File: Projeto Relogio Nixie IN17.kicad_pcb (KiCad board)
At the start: 2 copper layers, 50 x 50 mm, 73 parts, among them J1 nixie0, J2 nixie1, J3 BATTERY, J4 UART, P1 USB_C_Plug, Q1 BC817, Q2 STD17NF25, Q3 BC817, Q4 BC548, Q5 2N7000, Q6 BC548, Q7 BC548, Q8 BC548, SW1 SW_Push, SW2 SW_Push, SW3 SPST_B3U-1000P, SW4 SPST_B3U-1000P, U1 MAX1771xSA, U2 CP2102N-A01-GQFN24, U3 HV5523K7-G, U4 PAM2305AABADJ, U5 MCP73831-3-OT, U6 ESP32-PICO-D4

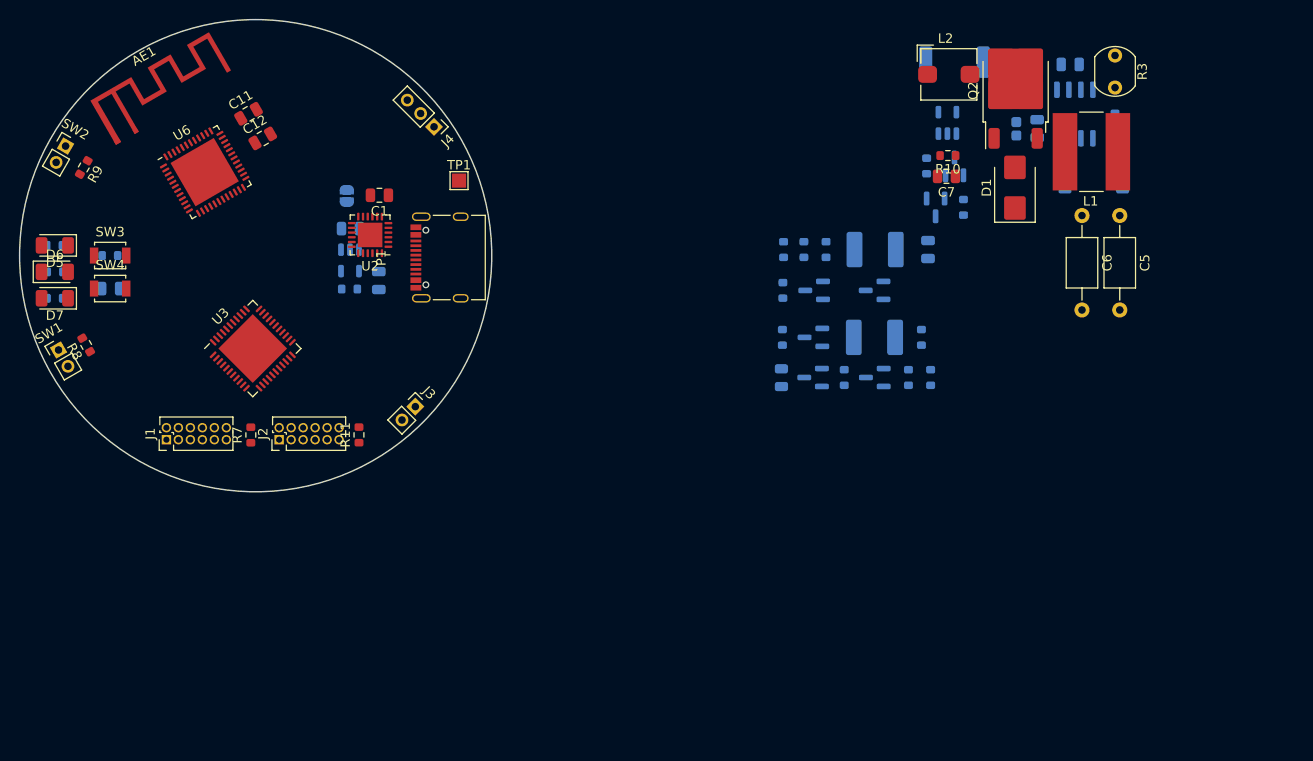
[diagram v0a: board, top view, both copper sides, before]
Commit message: Add files via upload
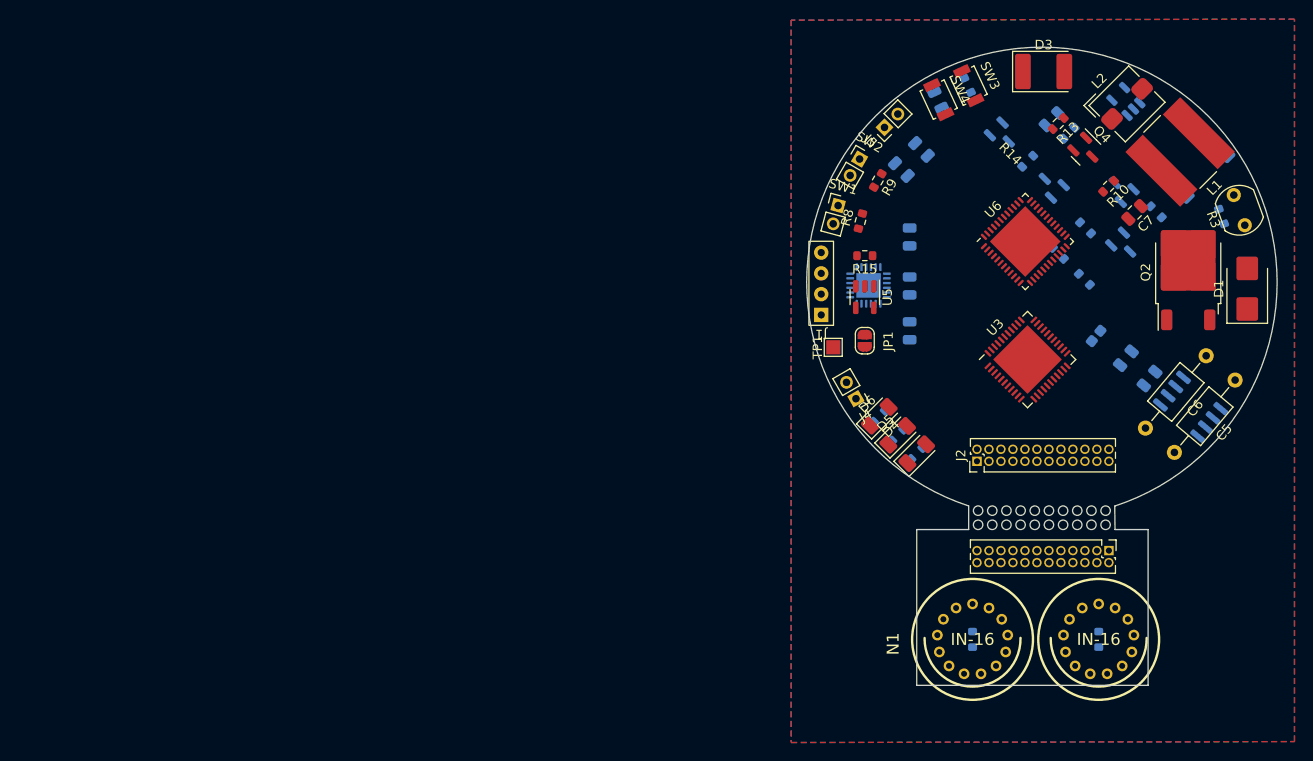
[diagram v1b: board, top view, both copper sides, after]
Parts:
- removed AE1: Antenna, ESP_Antenna:ESPRESSIF_ESP32_MIFA_2.4GHz_Right
- removed the C8 at (131.2, 58.4)
- removed the D4 at (125.5, 67.7)
- removed the J4 at (78.9, 45.4)
- removed P1: USB_C_Plug, Connector_USB:USB_C_Receptacle_Palconn_UTC16-G
- removed Q7, Q8: BC548, Package_TO_SOT_SMD:SOT-23
- removed the R15 at (115.8, 62.7)
- removed the R18 at (131.5, 71.9)
- removed the R19 at (118.0, 58.4)
- removed the R20 at (130.5, 67.7)
- removed the R21 at (120.4, 58.4)
- removed the R7 at (59.5, 78.0)
- added J3: Conn_01x24, Connector_PinHeader_1.27mm:PinHeader_2x12_P1.27mm_Vertical, F.Cu at (150.4, 90.2)
- added J5: ANTENNA, Connector_PinHeader_2.00mm:PinHeader_1x02_P2.00mm_Vertical, F.Cu at (126.6, 45.4)
- added N1: IN-16, nixies-us:nixies-us-IN-16, F.Cu at (135.9, 99.6)
- added N2: IN-16, nixies-us:nixies-us-IN-16, F.Cu at (149.3, 99.6)
- added R17: 100R, Resistor_SMD:R_0603_1608Metric, B.Cu at (147.8, 61.5)
- added R5: 15K, Resistor_SMD:R_0603_1608Metric, B.Cu at (135.9, 99.6)
- C1, R11, U2: moved to B.Cu
- C10: renamed from C11; moved to B.Cu
- C11: renamed from C12; moved to B.Cu
- D3: value DZ2S056X0L -> BZD27Cxx; moved to F.Cu
- J1: value nixie0 -> Conn_01x04; footprint Connector_PinHeader_1.27mm:PinHeader_2x06_P1.27mm_Vertical -> Connector:Magnetic_01x04
- J2: value nixie1 -> Conn_01x24; footprint Connector_PinHeader_1.27mm:PinHeader_2x06_P1.27mm_Vertical -> Connector_PinHeader_1.27mm:PinHeader_2x12_P1.27mm_Vertical
- JP1, Q4, R13, U5: moved to F.Cu
- Q5: value 2N7000 -> BC548
- R14: value 2K2 -> 1K
- R15: renamed from R17; moved to F.Cu
- moved R19 93.9 mm to (130.0, 79.9), turned to 45 degrees
- moved D4 93.9 mm to (130.0, 80.0), turned to 45 degrees
- moved SW3 92.7 mm to (135.5, 41.0), turned to -65 degrees
- moved R18 92.6 mm to (135.4, 41.0), turned to -65 degrees
- moved D5 90.9 mm to (128.0, 78.0), turned to 45 degrees
- moved R20 90.9 mm to (128.0, 78.0), turned to -135 degrees
- moved SW4 90.0 mm to (132.3, 42.5), turned to -65 degrees
- moved C12 89.9 mm to (132.2, 42.5), turned to -65 degrees
- moved D6 88.2 mm to (126.0, 76.0), turned to 45 degrees
- moved R21 88.2 mm to (126.0, 76.0), turned to -135 degrees
- moved U6 87.2 mm to (141.5, 57.5), turned to 45 degrees
- moved R9 84.1 mm to (125.9, 51.0)
- moved SW2 84.1 mm to (124.0, 48.8)
- moved SW1 84.0 mm to (121.7, 53.7), turned to -15 degrees
- moved R8 83.0 mm to (124.0, 55.3), turned to 75 degrees
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- renumbered C13 to C12, C9 to C8, C10 to C9, D5 to D4, D6 to D5, D7 to D6, J3 to J4, R22 to R18, R23 to R19, R24 to R20, R25 to R21, R5 to R6, R6 to R7
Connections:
- net IN1_6 renamed Net-(J2-Pin_7)
- D3 pad 2: BAT- -> Net-(D3-A)
- J1 pad 1: IN0_0 -> VIN
- J1 pad 2: IN0_1 -> RX0
- J1 pad 3: IN0_2 -> TX0
- J1 pad 4: IN0_3 -> BAT-
- J2 pad 1: IN1_0 -> HV
- J2 pad 10: IN1_9 -> Net-(J2-Pin_10)
- J2 pad 11: IN1_DP -> Net-(J2-Pin_11)
- J2 pad 2: IN1_1 -> HV
- J2 pad 3: IN1_2 -> Net-(J2-Pin_3)
- J2 pad 4: IN1_3 -> Net-(J2-Pin_4)
- J2 pad 5: IN1_4 -> Net-(J2-Pin_5)
- J2 pad 6: IN1_5 -> Net-(J2-Pin_6)
- J2 pad 8: IN1_7 -> Net-(J2-Pin_8)
- J2 pad 9: IN1_8 -> Net-(J2-Pin_9)
- Q5 pad 1: 5VA -> Net-(Q4-B)
- Q5 pad 2: Net-(Q5-G) -> Net-(Q5-B)
- Q5 pad 3: VIN -> BAT-
- Q6 pad 1: VIN -> Net-(Q6-C)
- Q6 pad 3: Net-(Q5-G) -> BAT-
- R11 pad 1: HV -> HVe
- R11 pad 2: Net-(J2-Pin_12) -> Net-(N2-PadA)
- R12 pad 2: Net-(Q8-C) -> Net-(Q6-C)
- R14 pad 1: VIN -> Net-(Q5-B)
- R14 pad 2: Net-(R14-Pad2) -> Net-(Q6-C)
- R16 pad 1: Net-(Q7-B) -> Net-(Q6-B)
- R16 pad 2: Net-(Q8-C) -> Net-(D3-A)
- U3 pad 1: IN0_0 -> Net-(J2-Pin_24)
- U3 pad 10: IN0_9 -> Net-(J2-Pin_15)
- U3 pad 11: IN0_DP -> Net-(J2-Pin_14)
- U3 pad 12: IN1_0 -> Net-(J2-Pin_13)
- U3 pad 13: IN1_1 -> Net-(J2-Pin_12)
- U3 pad 14: IN1_2 -> Net-(J2-Pin_11)
- U3 pad 15: IN1_3 -> Net-(J2-Pin_10)
- U3 pad 16: IN1_4 -> Net-(J2-Pin_9)
- U3 pad 17: IN1_5 -> Net-(J2-Pin_8)
- U3 pad 19: IN1_7 -> Net-(J2-Pin_6)
- U3 pad 2: IN0_1 -> Net-(J2-Pin_23)
- U3 pad 20: IN1_8 -> Net-(J2-Pin_5)
- U3 pad 21: IN1_9 -> Net-(J2-Pin_4)
- U3 pad 22: IN1_DP -> Net-(J2-Pin_3)
- U3 pad 3: IN0_2 -> Net-(J2-Pin_22)
- U3 pad 4: IN0_3 -> Net-(J2-Pin_21)
- U3 pad 5: IN0_4 -> Net-(J2-Pin_20)
- U3 pad 6: IN0_5 -> Net-(J2-Pin_19)
- U3 pad 7: IN0_6 -> Net-(J2-Pin_18)
- U3 pad 8: IN0_7 -> Net-(J2-Pin_17)
- U3 pad 9: IN0_8 -> Net-(J2-Pin_16)
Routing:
- added copper zone on B.Cu, net BAT-
- added copper zone on F.Cu, net BAT-
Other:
- board size 50 x 50 mm -> 49.8 x 67.6 mm
